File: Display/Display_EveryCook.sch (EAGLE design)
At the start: 127 parts

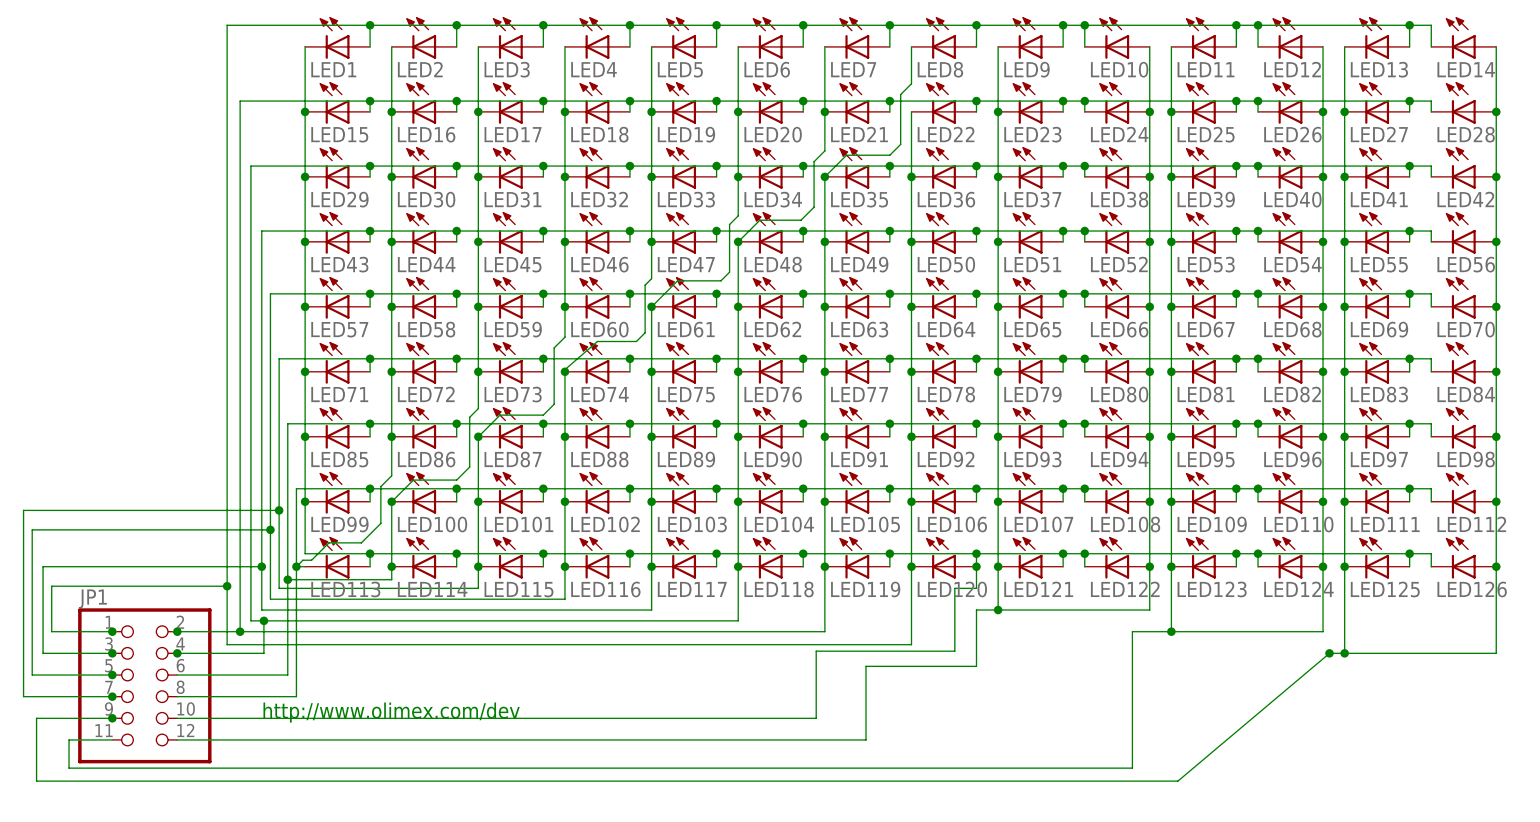
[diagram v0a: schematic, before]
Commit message: Redesign of all boards.
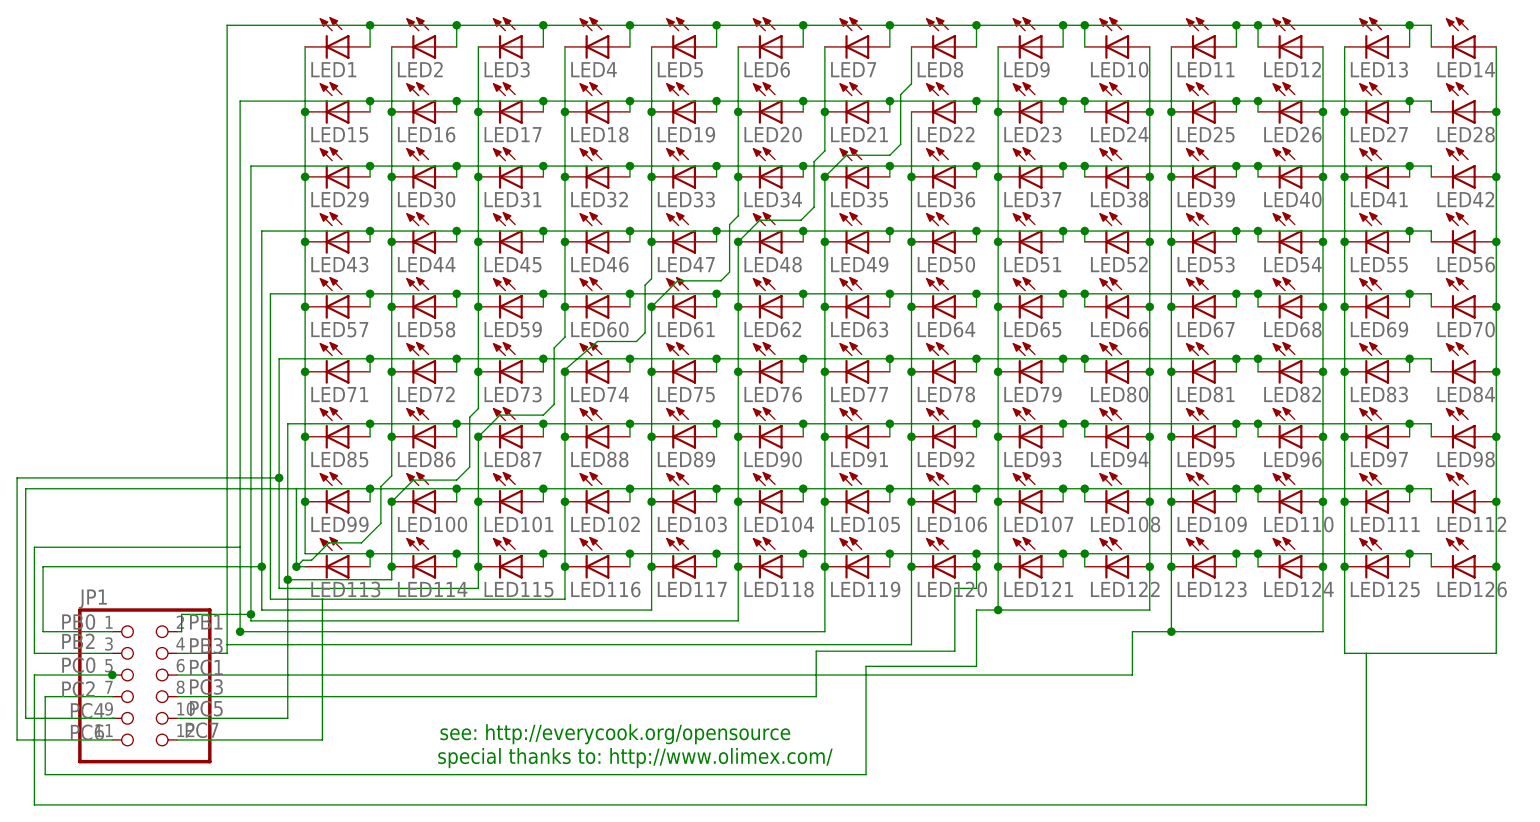
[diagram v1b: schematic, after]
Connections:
- removed net N$5: JP1.12, LED10.A, LED107.C, LED108.A, LED121.C, LED122.A, LED23.C, LED24.A, LED37.C, LED38.A, LED51.C, LED52.A, LED65.C, LED66.A, LED79.C, LED80.A, LED9.C, LED93.C, LED94.A
- removed net PIN10: JP1.3, LED103.C, LED117.C, LED20.C, LED34.C, LED43.A, LED44.A, LED45.A, LED46.A, LED47.A, LED48.A, LED49.A, LED50.A, LED51.A, LED52.C, LED53.A, LED54.C, LED55.A, LED56.C, LED6.C, LED61.C, LED75.C, LED89.C
- removed net PIN11: JP1.4, LED104.C, LED118.C, LED21.C, LED29.A, LED30.A, LED31.A, LED32.A, LED33.A, LED34.A, LED35.A, LED36.A, LED37.A, LED38.C, LED39.A, LED40.C, LED41.A, LED42.C, LED48.C, LED62.C, LED7.C, LED76.C, LED90.C
- removed net PIN12: JP1.2, LED105.C, LED119.C, LED15.A, LED16.A, LED17.A, LED18.A, LED19.A, LED20.A, LED21.A, LED22.A, LED23.A, LED24.C, LED25.A, LED26.C, LED27.A, LED28.C, LED35.C, LED49.C, LED63.C, LED77.C, LED8.C, LED91.C
- removed net PIN13: JP1.1, LED1.A, LED10.C, LED106.C, LED11.A, LED12.C, LED120.C, LED13.A, LED14.C, LED2.A, LED22.C, LED3.A, LED36.C, LED4.A, LED5.A, LED50.C, LED6.A, LED64.C, LED7.A, LED78.C, LED8.A, LED9.A, LED92.C
- removed net PIN2: JP1.9, LED111.C, LED112.A, LED125.C, LED126.A, LED13.C, LED14.A, LED27.C, LED28.A, LED41.C, LED42.A, LED55.C, LED56.A, LED69.C, LED70.A, LED83.C, LED84.A, LED97.C, LED98.A
- removed net PIN3: JP1.11, LED109.C, LED11.C, LED110.A, LED12.A, LED123.C, LED124.A, LED25.C, LED26.A, LED39.C, LED40.A, LED53.C, LED54.A, LED67.C, LED68.A, LED81.C, LED82.A, LED95.C, LED96.A
- removed net PIN5: JP1.10, LED1.C, LED113.A, LED114.A, LED115.A, LED116.A, LED117.A, LED118.A, LED119.A, LED120.A, LED121.A, LED122.C, LED123.A, LED124.C, LED125.A, LED126.C, LED15.C, LED29.C, LED43.C, LED57.C, LED71.C, LED85.C, LED99.C
- removed net PIN6: JP1.8, LED100.A, LED101.A, LED102.A, LED103.A, LED104.A, LED105.A, LED106.A, LED107.A, LED108.C, LED109.A, LED110.C, LED111.A, LED112.C, LED113.C, LED16.C, LED2.C, LED30.C, LED44.C, LED58.C, LED72.C, LED86.C, LED99.A
- removed net PIN7: JP1.6, LED100.C, LED114.C, LED17.C, LED3.C, LED31.C, LED45.C, LED59.C, LED73.C, LED85.A, LED86.A, LED87.A, LED88.A, LED89.A, LED90.A, LED91.A, LED92.A, LED93.A, LED94.C, LED95.A, LED96.C, LED97.A, LED98.C
- removed net PIN8: JP1.7, LED101.C, LED115.C, LED18.C, LED32.C, LED4.C, LED46.C, LED60.C, LED71.A, LED72.A, LED73.A, LED74.A, LED75.A, LED76.A, LED77.A, LED78.A, LED79.A, LED80.C, LED81.A, LED82.C, LED83.A, LED84.C, LED87.C
- removed net PIN9: JP1.5, LED102.C, LED116.C, LED19.C, LED33.C, LED47.C, LED5.C, LED57.A, LED58.A, LED59.A, LED60.A, LED61.A, LED62.A, LED63.A, LED64.A, LED65.A, LED66.C, LED67.A, LED68.C, LED69.A, LED70.C, LED74.C, LED88.C
- new net PB0: JP1.1, LED103.C, LED117.C, LED20.C, LED34.C, LED43.A, LED44.A, LED45.A, LED46.A, LED47.A, LED48.A, LED49.A, LED50.A, LED51.A, LED52.C, LED53.A, LED54.C, LED55.A, LED56.C, LED6.C, LED61.C, LED75.C, LED89.C
- new net PB1: JP1.2, LED104.C, LED118.C, LED21.C, LED29.A, LED30.A, LED31.A, LED32.A, LED33.A, LED34.A, LED35.A, LED36.A, LED37.A, LED38.C, LED39.A, LED40.C, LED41.A, LED42.C, LED48.C, LED62.C, LED7.C, LED76.C, LED90.C
- new net PB2: JP1.3, LED105.C, LED119.C, LED15.A, LED16.A, LED17.A, LED18.A, LED19.A, LED20.A, LED21.A, LED22.A, LED23.A, LED24.C, LED25.A, LED26.C, LED27.A, LED28.C, LED35.C, LED49.C, LED63.C, LED77.C, LED8.C, LED91.C
- new net PB3: JP1.4, LED1.A, LED10.C, LED106.C, LED11.A, LED12.C, LED120.C, LED13.A, LED14.C, LED2.A, LED22.C, LED3.A, LED36.C, LED4.A, LED5.A, LED50.C, LED6.A, LED64.C, LED7.A, LED78.C, LED8.A, LED9.A, LED92.C
- new net PC0: JP1.5, LED111.C, LED112.A, LED125.C, LED126.A, LED13.C, LED14.A, LED27.C, LED28.A, LED41.C, LED42.A, LED55.C, LED56.A, LED69.C, LED70.A, LED83.C, LED84.A, LED97.C, LED98.A
- new net PC1: JP1.6, LED109.C, LED11.C, LED110.A, LED12.A, LED123.C, LED124.A, LED25.C, LED26.A, LED39.C, LED40.A, LED53.C, LED54.A, LED67.C, LED68.A, LED81.C, LED82.A, LED95.C, LED96.A
- new net PC2: JP1.7, LED10.A, LED107.C, LED108.A, LED121.C, LED122.A, LED23.C, LED24.A, LED37.C, LED38.A, LED51.C, LED52.A, LED65.C, LED66.A, LED79.C, LED80.A, LED9.C, LED93.C, LED94.A
- new net PC3: JP1.8, LED1.C, LED113.A, LED114.A, LED115.A, LED116.A, LED117.A, LED118.A, LED119.A, LED120.A, LED121.A, LED122.C, LED123.A, LED124.C, LED125.A, LED126.C, LED15.C, LED29.C, LED43.C, LED57.C, LED71.C, LED85.C, LED99.C
- new net PC4: JP1.9, LED100.A, LED101.A, LED102.A, LED103.A, LED104.A, LED105.A, LED106.A, LED107.A, LED108.C, LED109.A, LED110.C, LED111.A, LED112.C, LED113.C, LED16.C, LED2.C, LED30.C, LED44.C, LED58.C, LED72.C, LED86.C, LED99.A
- new net PC5: JP1.10, LED100.C, LED114.C, LED17.C, LED3.C, LED31.C, LED45.C, LED59.C, LED73.C, LED85.A, LED86.A, LED87.A, LED88.A, LED89.A, LED90.A, LED91.A, LED92.A, LED93.A, LED94.C, LED95.A, LED96.C, LED97.A, LED98.C
- new net PC6: JP1.11, LED101.C, LED115.C, LED18.C, LED32.C, LED4.C, LED46.C, LED60.C, LED71.A, LED72.A, LED73.A, LED74.A, LED75.A, LED76.A, LED77.A, LED78.A, LED79.A, LED80.C, LED81.A, LED82.C, LED83.A, LED84.C, LED87.C
- new net PC7: JP1.12, LED102.C, LED116.C, LED19.C, LED33.C, LED47.C, LED5.C, LED57.A, LED58.A, LED59.A, LED60.A, LED61.A, LED62.A, LED63.A, LED64.A, LED65.A, LED66.C, LED67.A, LED68.C, LED69.A, LED70.C, LED74.C, LED88.C
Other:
- note added: "see: http://everycook.org/opensource"
- note added: "special thanks to: http://www.olimex.com/"
- note removed: "http://www.olimex.com/dev"
